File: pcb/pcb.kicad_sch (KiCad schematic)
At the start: 153 parts, among them J1 USB_C_Receptacle_USB2.0_14P, SW0 SW_Push, SW1 SW_Push_45deg, SW10 SW_Push_45deg, SW11 SW_Push_45deg, SW12 SW_Push_45deg, SW13 SW_Push_45deg, SW14 SW_Push_45deg, SW15 SW_Push_45deg, SW16 SW_Push_45deg, SW17 SW_Push_45deg, SW18 SW_Push_45deg, SW19 SW_Push_45deg, SW2 SW_Push_45deg, SW20 SW_Push_45deg, SW21 SW_Push_45deg, SW22 SW_Push_45deg, SW23 SW_Push_45deg, SW24 SW_Push_45deg, SW25 SW_Push_45deg, SW26 SW_Push_45deg, SW27 SW_Push_45deg, SW28 SW_Push_45deg, SW29 SW_Push_45deg, SW3 SW_Push_45deg, SW30 SW_Push_45deg, SW31 SW_Push_45deg, SW32 SW_Push_45deg, SW33 SW_Push_45deg, SW34 SW_Push_45deg, SW35 SW_Push_45deg, SW36 SW_Push_45deg, SW37 SW_Push_45deg, SW38 SW_Push_45deg, SW39 SW_Push_45deg, SW4 SW_Push_45deg, SW40 SW_Push_45deg, SW41 SW_Push_45deg, SW42 SW_Push_45deg, SW43 SW_Push_45deg, SW44 SW_Push_45deg, SW45 SW_Push_45deg, SW46 SW_Push_45deg, SW47 SW_Push_45deg, SW48 SW_Push_45deg, SW49 SW_Push_45deg, SW5 SW_Push_45deg, SW50 SW_Push_45deg, SW51 SW_Push_45deg, SW52 SW_Push_45deg, SW53 SW_Push_45deg, SW54 SW_Push_45deg, SW55 SW_Push_45deg, SW56 SW_Push_45deg, SW57 SW_Push_45deg, SW58 SW_Push_45deg, SW59 SW_Push_45deg, SW6 SW_Push_45deg, SW60 SW_Push_45deg, SW61 SW_Push_45deg, SW62 SW_Push_45deg, SW63 SW_Push_45deg, SW64 SW_Push_45deg, SW65 SW_Push_45deg, SW66 SW_Push_45deg, SW67 SW_Push_45deg, SW68 SW_Push_45deg, SW7 SW_Push_45deg, SW8 SW_Push_45deg, SW9 SW_Push_45deg, U1 ATmega32U4-A, Y1 16MHz

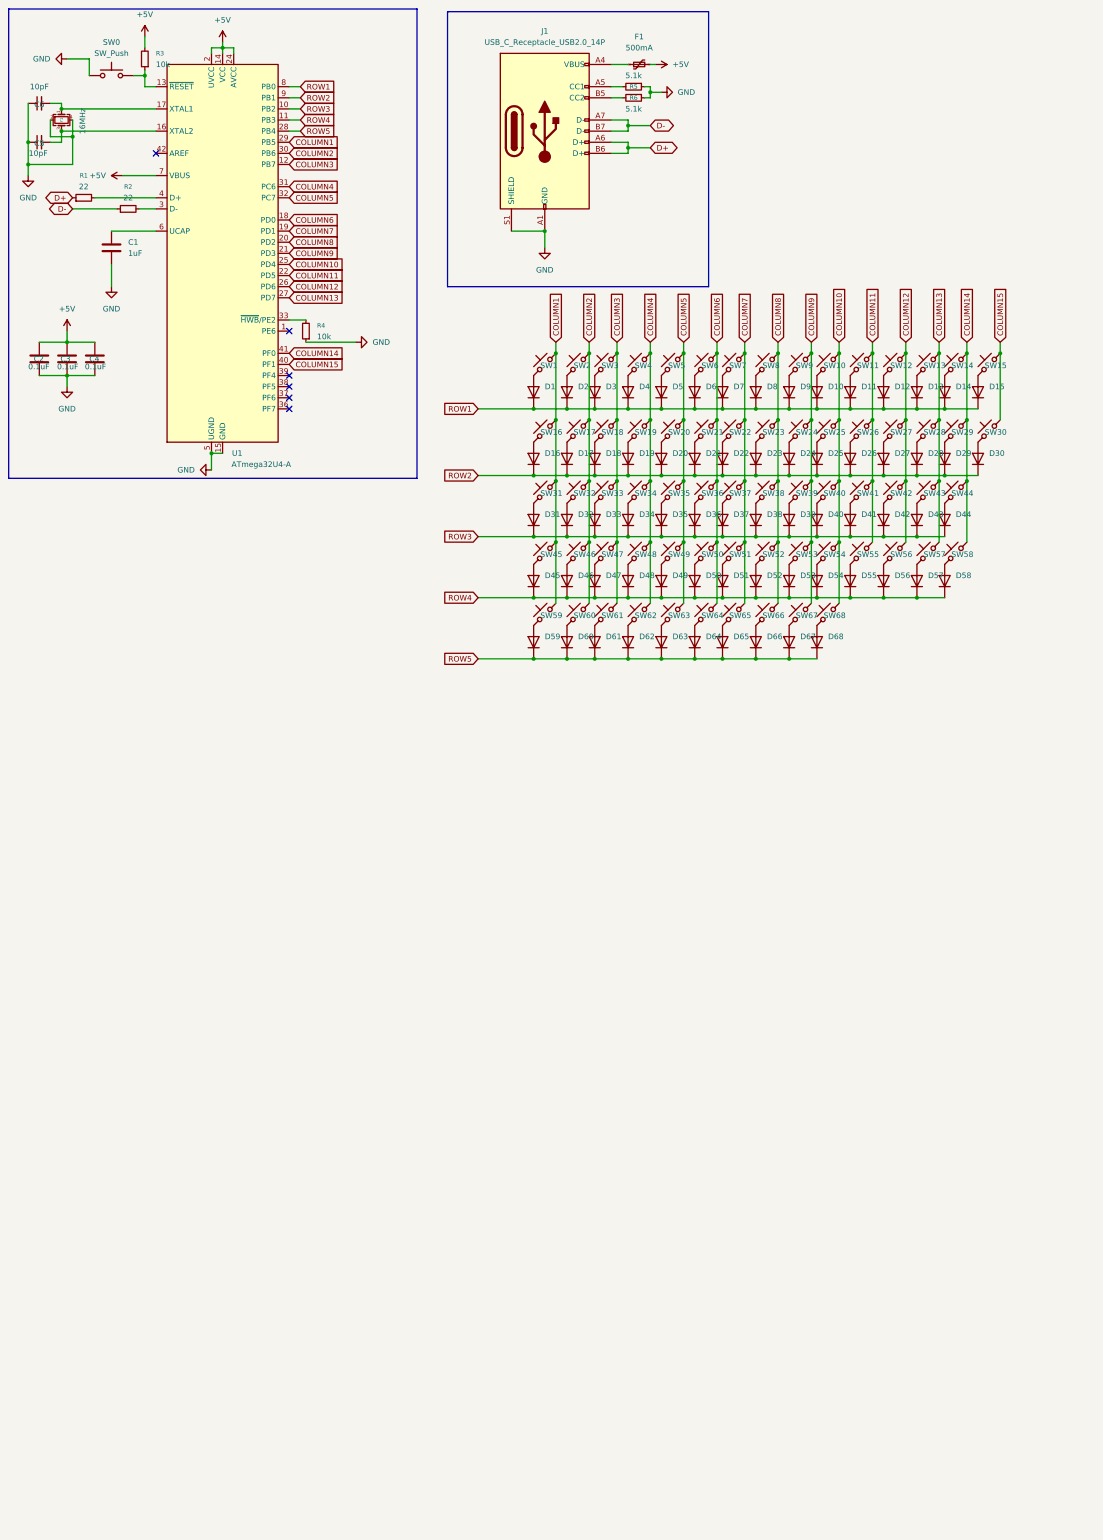
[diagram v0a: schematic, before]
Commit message: Initial Commit
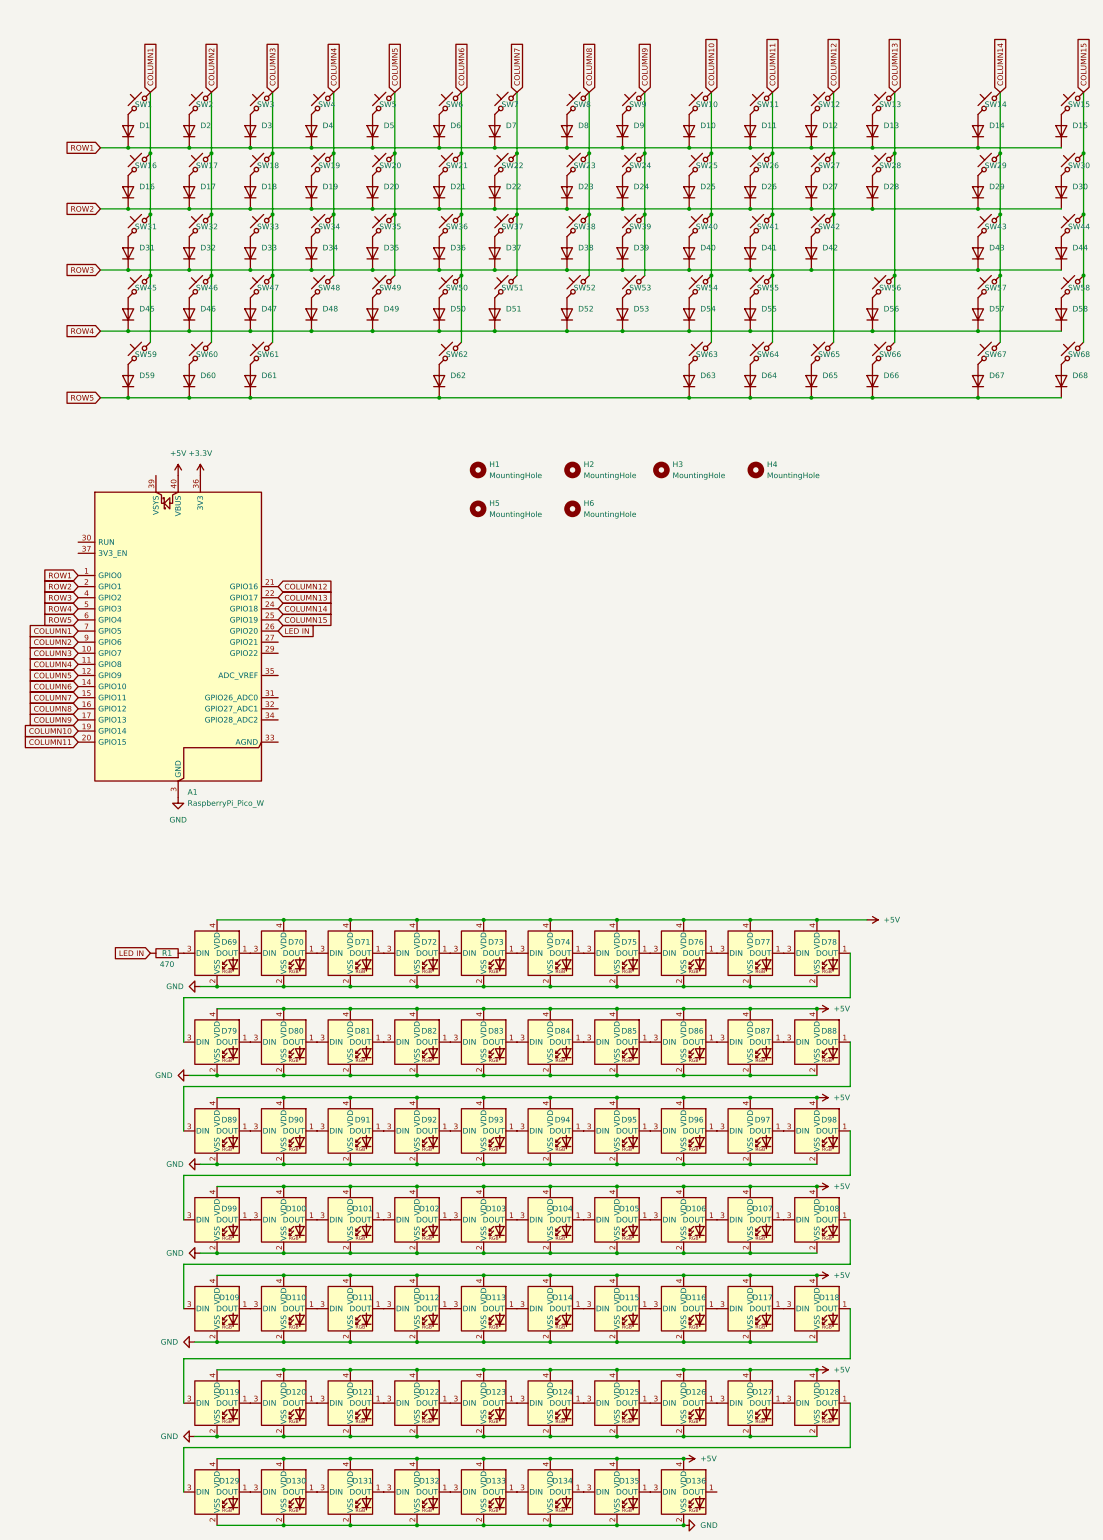
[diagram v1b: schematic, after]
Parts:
- removed C1: 1uF, Capacitor_SMD:C_0805_2012Metric, symbol Device:C
- removed C2, C3, C4: 0.1uF, Capacitor_SMD:C_0805_2012Metric, symbol Device:C
- removed C5, C6: 10pF, Capacitor_SMD:C_0805_2012Metric, symbol Device:C_Small
- removed F1: 500mA, Fuse:Fuse_1206_3216Metric, symbol Device:Polyfuse_Small
- removed J1: USB_C_Receptacle_USB2.0_14P, Connector_USB:USB_C_Receptacle_Amphenol_12401548E4-2A, symbol Connector:USB_C_Receptacle_USB2.0_14P
- removed R1, R2: 22, Resistor_SMD:R_0805_2012Metric, symbol Device:R_Small
- removed R3, R4: 10k, Resistor_SMD:R_0805_2012Metric, symbol Device:R_Small
- removed R5, R6: 5.1k, Resistor_SMD:R_0805_2012Metric, symbol Device:R_Small
- removed SW0: SW_Push, Button_Switch_SMD:SW_SPST_B3S-1000, symbol Switch:SW_Push
- removed U1: ATmega32U4-A, Package_QFP:TQFP-44_10x10mm_P0.8mm, symbol MCU_Microchip_ATmega:ATmega32U4-A
- removed Y1: 16MHz, Crystal:Crystal_SMD_3225-4Pin_3.2x2.5mm, symbol Device:Crystal_GND24_Small
- added A1: RaspberryPi_Pico_W, Module:RaspberryPi_Pico_Common_THT, symbol MCU_Module:RaspberryPi_Pico_W
- added D100, D101, D102, D103, D104, D105, D106, D107, D108, D109, D110, D111, D112, D113, D114, D115, D116, D117, D118, D119, D120, D121, D122, D123, D124, D125, D126, D127, D128, D129, D130, D131, D132, D133, D134, D135, D136, D69, D70, D71, D72, D73, D74, D75, D76, D77, D78, D79, D80, D81, D82, D83, D84, D85, D86, D87, D88, D89, D90, D91, D92, D93, D94, D95, D96, D97, D98, D99: SK6812MINI, KEYS:MX_SK6812MINI-E, symbol LED:SK6812MINI
- added H1, H2, H3, H4, H5, H6: MountingHole, MountingHole:MountingHole_3.2mm_M3, symbol Mechanical:MountingHole
- added R1: 470, Resistor_THT:R_Axial_DIN0614_L14.3mm_D5.7mm_P20.32mm_Horizontal, symbol Device:R
- SW1, SW10, SW11, SW12, SW13, SW17, SW18, SW19, SW2, SW20, SW21, SW22, SW23, SW24, SW25, SW26, SW27, SW28, SW3, SW32, SW33, SW34, SW35, SW36, SW37, SW38, SW39, SW4, SW40, SW41, SW42, SW46, SW47, SW48, SW49, SW5, SW50, SW51, SW52, SW53, SW54, SW55, SW57, SW58, SW6, SW7, SW8, SW9: footprint Button_Switch_Keyboard:SW_Cherry_MX_1.00u_PCB -> KEYS:SW_Hotswap_Kailh_MX_1.00u
- SW14: footprint Button_Switch_Keyboard:SW_Cherry_MX_1.00u_PCB -> KEYS:SW_Hotswap_Kailh_MX_Plated_2.00u
- SW15: footprint Button_Switch_Keyboard:SW_Cherry_MX_2.00u_PCB -> KEYS:SW_Hotswap_Kailh_MX_1.00u
- SW16: footprint Button_Switch_Keyboard:SW_Cherry_MX_1.50u_PCB -> KEYS:SW_Hotswap_Kailh_MX_Plated_1.50u
- SW29: footprint Button_Switch_Keyboard:SW_Cherry_MX_1.00u_PCB -> KEYS:SW_Hotswap_Kailh_MX_Plated_1.50u
- SW30: footprint Button_Switch_Keyboard:SW_Cherry_MX_1.50u_PCB -> KEYS:SW_Hotswap_Kailh_MX_1.00u
- SW31, SW56: footprint Button_Switch_Keyboard:SW_Cherry_MX_1.75u_PCB -> KEYS:SW_Hotswap_Kailh_MX_Plated_1.75u
- SW43: footprint Button_Switch_Keyboard:SW_Cherry_MX_1.00u_PCB -> KEYS:SW_Hotswap_Kailh_MX_Plated_2.25u
- SW44: footprint Button_Switch_Keyboard:SW_Cherry_MX_2.25u_PCB -> KEYS:SW_Hotswap_Kailh_MX_1.00u
- SW45: footprint Button_Switch_Keyboard:SW_Cherry_MX_2.25u_PCB -> KEYS:SW_Hotswap_Kailh_MX_Plated_2.25u
- SW59, SW60, SW61: footprint Button_Switch_Keyboard:SW_Cherry_MX_1.00u_Plate -> KEYS:SW_Hotswap_Kailh_MX_Plated_1.25u
- SW62: footprint Button_Switch_Keyboard:SW_Cherry_MX_6.25u_PCB -> KEYS:SW_Hotswap_Kailh_MX_Plated_6.25u
- SW63, SW64, SW65, SW66, SW67, SW68: footprint Button_Switch_Keyboard:SW_Cherry_MX_1.00u_Plate -> KEYS:SW_Hotswap_Kailh_MX_1.00u
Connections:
- net +5V: now also A1.40 (VBUS), D100.4 (VDD), D101.4 (VDD), D102.4 (VDD), D103.4 (VDD), D104.4 (VDD), D105.4 (VDD), D106.4 (VDD), D107.4 (VDD), D108.4 (VDD), D109.4 (VDD), D110.4 (VDD), D111.4 (VDD), D112.4 (VDD), D113.4 (VDD), D114.4 (VDD), D115.4 (VDD), D116.4 (VDD), D117.4 (VDD), D118.4 (VDD), D119.4 (VDD), D120.4 (VDD), D121.4 (VDD), D122.4 (VDD), D123.4 (VDD), D124.4 (VDD), D125.4 (VDD), D126.4 (VDD), D127.4 (VDD), D128.4 (VDD), D129.4 (VDD), D130.4 (VDD), D131.4 (VDD), D132.4 (VDD), D133.4 (VDD), D134.4 (VDD), D135.4 (VDD), D136.4 (VDD), D69.4 (VDD), D70.4 (VDD), D71.4 (VDD), D72.4 (VDD), D73.4 (VDD), D74.4 (VDD), D75.4 (VDD), D76.4 (VDD), D77.4 (VDD), D78.4 (VDD), D79.4 (VDD), D80.4 (VDD), D81.4 (VDD), D82.4 (VDD), D83.4 (VDD), D84.4 (VDD), D85.4 (VDD), D86.4 (VDD), D87.4 (VDD), D88.4 (VDD), D89.4 (VDD), D90.4 (VDD), D91.4 (VDD), D92.4 (VDD), D93.4 (VDD), D94.4 (VDD), D95.4 (VDD), D96.4 (VDD), D97.4 (VDD), D98.4 (VDD), D99.4 (VDD)
- net COLUMN1: now also A1.7 (GPIO5)
- net COLUMN10: now also SW63.2, A1.19 (GPIO14); no longer SW68.2
- net COLUMN11: now also SW64.2, A1.20 (GPIO15)
- net COLUMN12: now also SW65.2, A1.21 (GPIO16); no longer SW56.2
- net COLUMN13: now also SW56.2, SW66.2, A1.22 (GPIO17); no longer SW43.2, SW57.2
- net COLUMN14: now also SW43.2, SW57.2, SW67.2, A1.24 (GPIO18); no longer SW44.2, SW58.2
- net COLUMN15: now also SW44.2, SW58.2, SW68.2, A1.25 (GPIO19)
- net COLUMN2: now also A1.9 (GPIO6)
- net COLUMN3: now also A1.10 (GPIO7)
- net COLUMN4: now also A1.11 (GPIO8); no longer SW62.2
- net COLUMN5: now also A1.12 (GPIO9); no longer SW63.2
- net COLUMN6: now also SW62.2, A1.14 (GPIO10); no longer SW64.2
- net COLUMN7: now also A1.15 (GPIO11); no longer SW65.2
- net COLUMN8: now also A1.16 (GPIO12); no longer SW66.2
- net COLUMN9: now also A1.17 (GPIO13); no longer SW67.2
- net GND: now also A1.13 (GND), A1.18 (GND), A1.23 (GND), A1.28 (GND), A1.3 (GND), A1.38 (GND), A1.8 (GND), D100.2 (VSS), D101.2 (VSS), D102.2 (VSS), D103.2 (VSS), D104.2 (VSS), D105.2 (VSS), D106.2 (VSS), D107.2 (VSS), D108.2 (VSS), D109.2 (VSS), D110.2 (VSS), D111.2 (VSS), D112.2 (VSS), D113.2 (VSS), D114.2 (VSS), D115.2 (VSS), D116.2 (VSS), D117.2 (VSS), D118.2 (VSS), D119.2 (VSS), D120.2 (VSS), D121.2 (VSS), D122.2 (VSS), D123.2 (VSS), D124.2 (VSS), D125.2 (VSS), D126.2 (VSS), D127.2 (VSS), D128.2 (VSS), D129.2 (VSS), D130.2 (VSS), D131.2 (VSS), D132.2 (VSS), D133.2 (VSS), D134.2 (VSS), D135.2 (VSS), D136.2 (VSS), D69.2 (VSS), D70.2 (VSS), D71.2 (VSS), D72.2 (VSS), D73.2 (VSS), D74.2 (VSS), D75.2 (VSS), D76.2 (VSS), D77.2 (VSS), D78.2 (VSS), D79.2 (VSS), D80.2 (VSS), D81.2 (VSS), D82.2 (VSS), D83.2 (VSS), D84.2 (VSS), D85.2 (VSS), D86.2 (VSS), D87.2 (VSS), D88.2 (VSS), D89.2 (VSS), D90.2 (VSS), D91.2 (VSS), D92.2 (VSS), D93.2 (VSS), D94.2 (VSS), D95.2 (VSS), D96.2 (VSS), D97.2 (VSS), D98.2 (VSS), D99.2 (VSS)
- net ROW1: now also A1.1 (GPIO0)
- net ROW2: now also A1.2 (GPIO1)
- net ROW3: now also A1.4 (GPIO2)
- net ROW4: now also A1.5 (GPIO3)
- net ROW5: now also A1.6 (GPIO4)
- new net: D98.1 (DOUT), D99.3 (DIN)
- new net: D97.1 (DOUT), D98.3 (DIN)
- new net: D100.1 (DOUT), D101.3 (DIN)
- new net: D100.3 (DIN), D99.1 (DOUT)
- new net: D124.1 (DOUT), D125.3 (DIN)
- new net: D123.1 (DOUT), D124.3 (DIN)
- new net: D127.1 (DOUT), D128.3 (DIN)
- new net: D126.1 (DOUT), D127.3 (DIN)
- new net: D128.1 (DOUT), D129.3 (DIN)
- new net: D121.1 (DOUT), D122.3 (DIN)
- new net: D120.1 (DOUT), D121.3 (DIN)
- new net: D87.1 (DOUT), D88.3 (DIN)
- new net: D86.1 (DOUT), D87.3 (DIN)
- new net: D129.1 (DOUT), D130.3 (DIN)
- new net: D114.1 (DOUT), D115.3 (DIN)
- new net: D113.1 (DOUT), D114.3 (DIN)
- new net: D101.1 (DOUT), D102.3 (DIN)
- new net: D103.1 (DOUT), D104.3 (DIN)
- new net: D102.1 (DOUT), D103.3 (DIN)
- new net: D130.1 (DOUT), D131.3 (DIN)
- new net: D122.1 (DOUT), D123.3 (DIN)
- new net: D125.1 (DOUT), D126.3 (DIN)
- new net: D133.1 (DOUT), D134.3 (DIN)
- new net: D132.1 (DOUT), D133.3 (DIN)
- new net: D105.1 (DOUT), D106.3 (DIN)
- new net: D104.1 (DOUT), D105.3 (DIN)
- new net: D111.1 (DOUT), D112.3 (DIN)
- new net: D110.1 (DOUT), D111.3 (DIN)
- new net: D84.1 (DOUT), D85.3 (DIN)
- new net: D83.1 (DOUT), D84.3 (DIN)
- new net: D135.1 (DOUT), D136.3 (DIN)
- new net: D134.1 (DOUT), D135.3 (DIN)
- new net: D116.1 (DOUT), D117.3 (DIN)
- new net: D115.1 (DOUT), D116.3 (DIN)
- new net: D109.1 (DOUT), D110.3 (DIN)
- new net: D108.1 (DOUT), D109.3 (DIN)
- new net: D88.1 (DOUT), D89.3 (DIN)
- new net: D96.1 (DOUT), D97.3 (DIN)
- new net: D95.1 (DOUT), D96.3 (DIN)
- new net: D119.1 (DOUT), D120.3 (DIN)
- new net: D118.1 (DOUT), D119.3 (DIN)
- new net: D106.1 (DOUT), D107.3 (DIN)
- new net: D93.1 (DOUT), D94.3 (DIN)
- new net: D92.1 (DOUT), D93.3 (DIN)
- new net: D78.1 (DOUT), D79.3 (DIN)
- new net: D77.1 (DOUT), D78.3 (DIN)
- new net: D107.1 (DOUT), D108.3 (DIN)
- new net: D82.1 (DOUT), D83.3 (DIN)
- new net: D91.1 (DOUT), D92.3 (DIN)
- new net: D69.3 (DIN), R1.2
- new net: D117.1 (DOUT), D118.3 (DIN)
- new net: D94.1 (DOUT), D95.3 (DIN)
- new net: D90.1 (DOUT), D91.3 (DIN)
- new net: D89.1 (DOUT), D90.3 (DIN)
- new net: D71.1 (DOUT), D72.3 (DIN)
- new net: D70.1 (DOUT), D71.3 (DIN)
- new net: D69.1 (DOUT), D70.3 (DIN)
- new net: D85.1 (DOUT), D86.3 (DIN)
- new net: D112.1 (DOUT), D113.3 (DIN)
- new net: D81.1 (DOUT), D82.3 (DIN)
- new net: D131.1 (DOUT), D132.3 (DIN)
- new net: D73.1 (DOUT), D74.3 (DIN)
- new net: D72.1 (DOUT), D73.3 (DIN)
- new net: D74.1 (DOUT), D75.3 (DIN)
- new net: D75.1 (DOUT), D76.3 (DIN)
- new net: D80.1 (DOUT), D81.3 (DIN)
- new net: D76.1 (DOUT), D77.3 (DIN)
- new net: D79.1 (DOUT), D80.3 (DIN)
- new net +3.3V: A1.36 (3V3)
- new net LED IN: A1.26 (GPIO20), R1.1
- no-connect marks 6 -> 0
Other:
- moved on the sheet: D1, SW1
